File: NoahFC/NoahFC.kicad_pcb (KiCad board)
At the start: 2 copper layers, 36 x 56 mm, 54 parts, among them J1 ALE, J10 GND, J11 SCK, J12 MISO, J13 VCC, J14 GND, J16 CAM, J17 VTX, J18 RESET, J2 ELE, J4 FTDI, J5 VCC, J6 THR, J7 PPM, J8 GPS, U1 ATmega328, U2 MPU-6050, U3 AMS1117-5.0, U4 AMS1117-3.3, U5 MAX7456EUI+, U6 HMC5883L, Y1 16Mhz, Y2 27Mhz

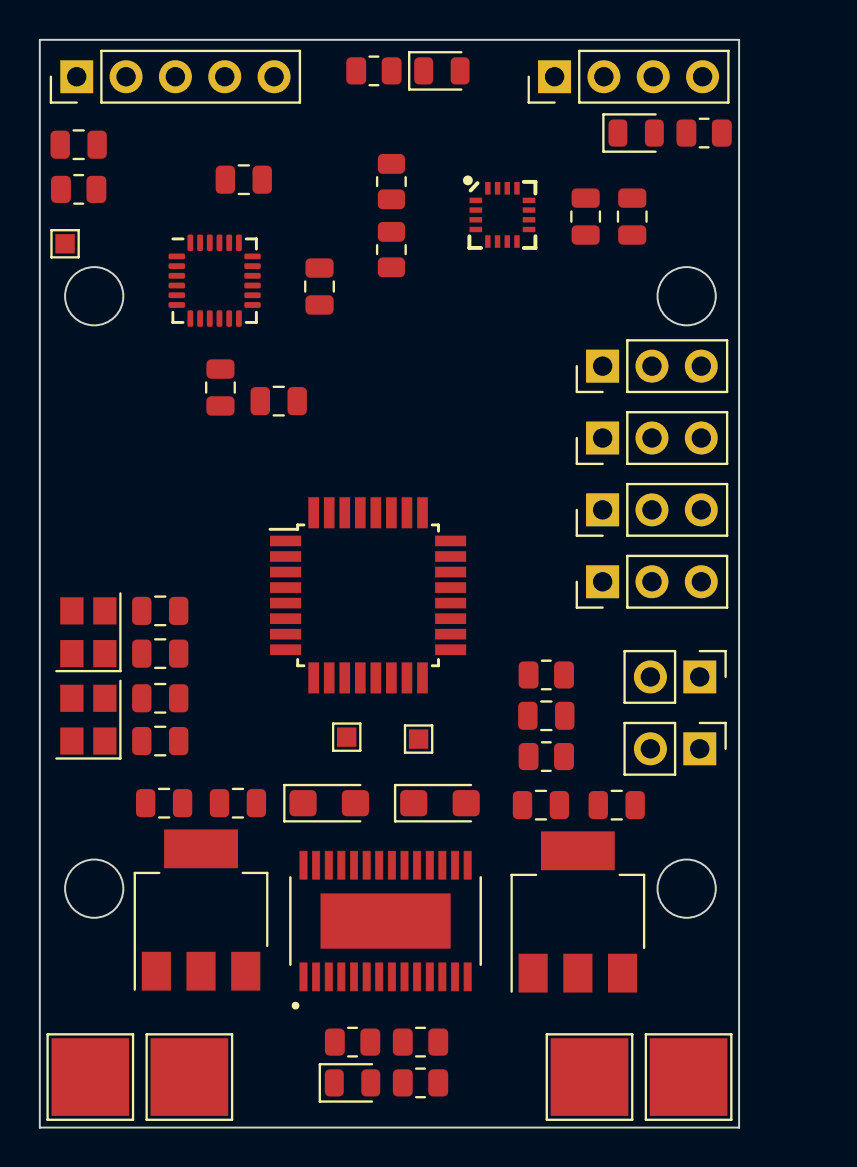
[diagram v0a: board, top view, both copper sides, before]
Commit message: update scheme / design and board
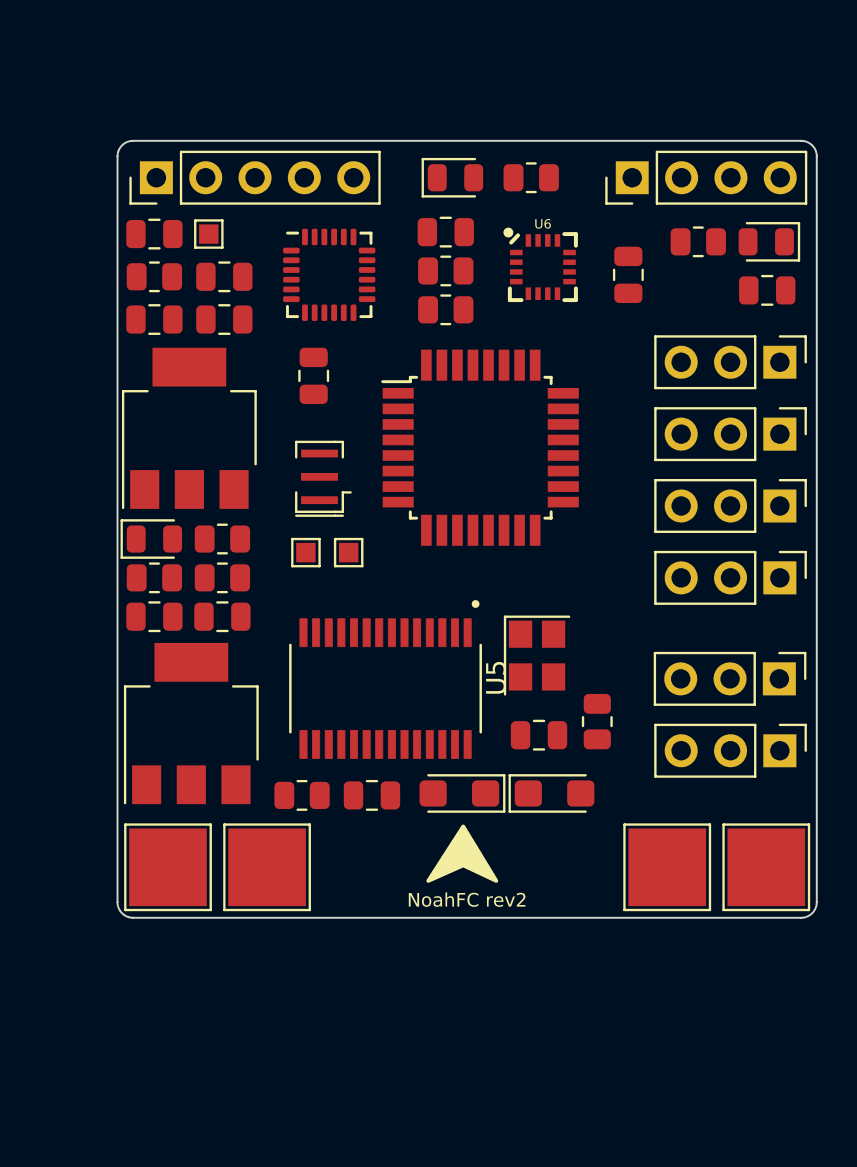
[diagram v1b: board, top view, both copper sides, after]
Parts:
- removed C1, C12, C13, C2: 22pF, Capacitor_SMD:C_0805_2012Metric
- removed J16: CAM, Connector_PinHeader_2.54mm:PinHeader_1x02_P2.54mm_Vertical
- added J3: CAM, Connector_PinHeader_2.54mm:PinHeader_1x03_P2.54mm_Vertical, F.Cu at (152.0, 106.1)
- C9: value 2200pF -> 2.2nF
- J17: footprint Connector_PinHeader_2.54mm:PinHeader_1x02_P2.54mm_Vertical -> Connector_PinHeader_2.54mm:PinHeader_1x03_P2.54mm_Vertical
- Y1: footprint Crystal:Crystal_SMD_3225-4Pin_3.2x2.5mm -> Crystal:Resonator_SMD_Murata_CSTxExxV-3Pin_3.0x1.1mm
- moved C10 34.5 mm to (119.8, 83.9), turned to 180 degrees
- moved U4 31.9 mm to (121.6, 89.5)
- moved C11 29.8 mm to (123.4, 83.9)
- moved D3 29.8 mm to (119.8, 95.2)
- moved R4 29.4 mm to (119.8, 97.2), turned to 0 degrees
- moved R6 27.8 mm to (123.3, 95.2)
- moved C7 25.7 mm to (139.6, 105.3), turned to 0 degrees
- moved R5 24.8 mm to (123.3, 97.2), turned to 180 degrees
- moved Y2 23.3 mm to (139.5, 101.2), turned to -90 degrees
- moved Y1 14.3 mm to (128.3, 92.0)
- moved R9 12.7 mm to (127.4, 108.4), turned to 180 degrees
- moved U5 12.0 mm to (131.7, 102.9), turned to -90 degrees
- moved C19 11.6 mm to (140.4, 108.3)
- moved J10 11.5 mm to (151.3, 112.1)
- moved J13 11.5 mm to (125.6, 112.1)
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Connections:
- J1 pad 1: ALERON -> GND_BEC
- J1 pad 3: GND_BEC -> ALERON
- J17 pad 2: Net-(J17-Pad2) -> unconnected-(J17-Pad2)
- J2 pad 1: ELEVATOR -> GND_BEC
- J2 pad 3: GND_BEC -> ELEVATOR
- J6 pad 1: THROTTLE -> GND_BEC
- J6 pad 3: GND_BEC -> THROTTLE
- J7 pad 1: PPM -> GND_BEC
- J7 pad 2: 5V -> 5V_BEC
- J7 pad 3: GND -> PPM
- R10 pad 2: Net-(J17-Pad2) -> Net-(R10-Pad2)
- Y1 pad 2: XTAL1 -> GND
- Y1 pad 3: (no net) -> XTAL1
- Y2 pad 2: XTAL2_OSD -> GND
- Y2 pad 3: (no net) -> XTAL2_OSD
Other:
- board size 36 x 56 mm -> 36 x 40 mm
- board text added: "NoahFC rev2"
- board text removed: "5V"
- board text removed: "DTR"
- board text removed: "GND"
- board text removed: "RX"
- board text removed: "SCL"
- board text removed: "SDA"
- board text removed: "TX"
